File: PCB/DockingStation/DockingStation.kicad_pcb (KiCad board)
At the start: 4 copper layers, 147.2 x 63.2 mm, 256 parts, among them CN1 DSUB-15-HD_Socket_Horizontal_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, CN2 FDC_Connector, CN4 DSUB-25_Socket_Horizontal_P2.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, CN5 DSUB-9_Pins_Horizontal_P2.77x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, CN6 PS2 Connector, CN7 PS2 Connector, CN8 BarrelJack_Horizontal_PC110, J1 PCB Edge, J2 PCB Edge, J3 PCB Edge, J4 PCB Edge, Q1 3P4J, Q2 8C, U1 74VHCT244, U2 DNP (LT1237CS), U3 DS14C535MSA, U4 DNP

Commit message: Add files via upload
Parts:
- J1, J2, J3, J4: value PCB Edge -> 25-1MP_P0.5mm_Horizontal
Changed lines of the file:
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@@
 			)
 		)
-		(property "Value" "PCB Edge"
+		(property "Value" "25-1MP_P0.5mm_Horizontal"
 			(at 0 -3.25 0)
 			(layer "Dwgs.User")
@@
 			)
 		)
-		(property "Value" "PCB Edge"
+		(property "Value" "25-1MP_P0.5mm_Horizontal"
 			(at 0 -3.25 0)
 			(layer "Dwgs.User")
@@
 			)
 		)
-		(property "Value" "PCB Edge"
+		(property "Value" "25-1MP_P0.5mm_Horizontal"
 			(at 0 -3.25 0)
 			(layer "Dwgs.User")
@@
 			)
 		)
-		(property "Value" "PCB Edge"
+		(property "Value" "25-1MP_P0.5mm_Horizontal"
 			(at 0 -3.25 0)
 			(layer "Dwgs.User")

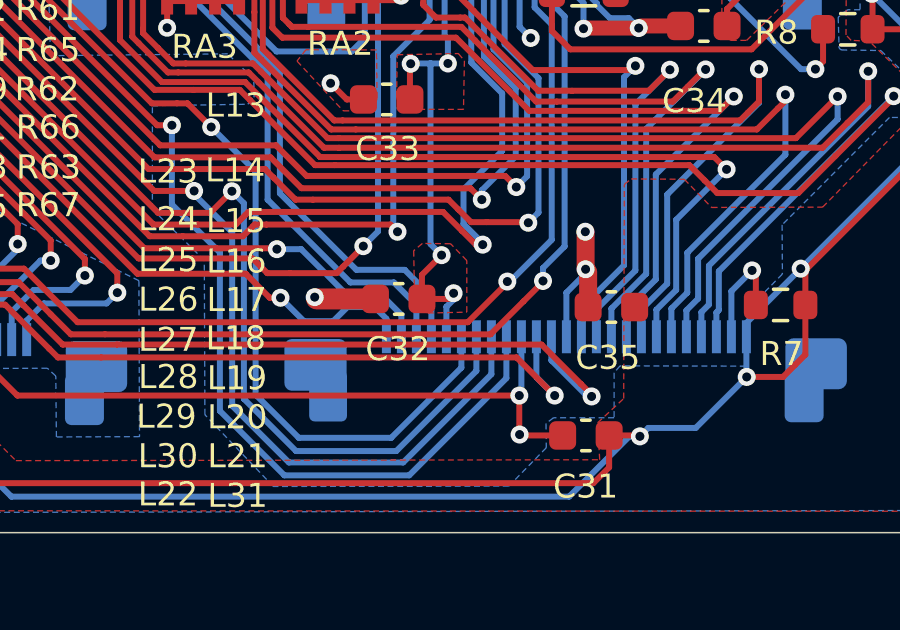
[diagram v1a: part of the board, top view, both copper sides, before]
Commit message: Add files via upload
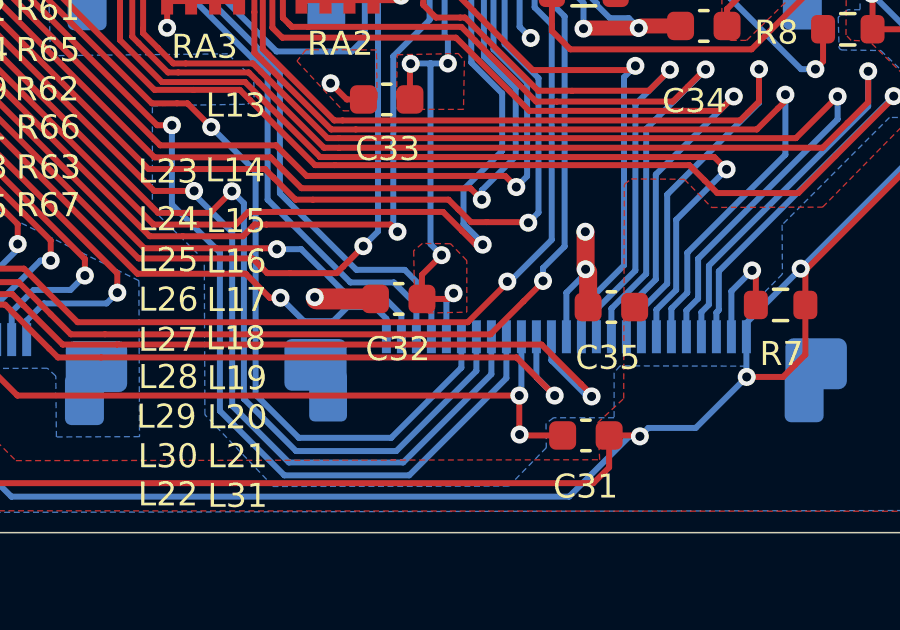
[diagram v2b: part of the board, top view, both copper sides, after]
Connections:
- net PNET1_Dock renamed PNET2
- net PNET2_Dock renamed PNET5
- C31 pad 2: (no net) -> PNET5_Q1_F2
- DA1 pad 3: (no net) -> VGA_RED
- DA2 pad 3: (no net) -> VGA_GREEN
- DA3 pad 3: (no net) -> VGA_BLUE
- J1 pad 11: (no net) -> VGA_BLUE
- J1 pad 13: (no net) -> R269_1_PC110
- J1 pad 14: (no net) -> M38_P16_R80_PC110
- J1 pad 15: (no net) -> M38_P67
- J1 pad 16: (no net) -> J13_60_PC110
- J1 pad 17: (no net) -> J13_59_PC110
- J1 pad 18: (no net) -> J13_58_PC110
- J1 pad 2: (no net) -> FDC_SLCTIN#
- J1 pad 24: (no net) -> J13_52_PC110
- J1 pad 3: (no net) -> FDC_AUTOFD#
- J1 pad 4: (no net) -> FDC_INIT#
- J1 pad 5: (no net) -> FDC_ACK#
- J1 pad 7: (no net) -> VGA_RED
- J1 pad 9: (no net) -> VGA_GREEN
- J2 pad 10: (no net) -> FDC_RDATA#
- J2 pad 11: (no net) -> J13_90_PC110
- J2 pad 14: (no net) -> KB_INT4
- J2 pad 15: (no net) -> KB_INT3
- J2 pad 17: (no net) -> FDC_DSR2#
- J2 pad 18: (no net) -> FDC_RTS2#
- J2 pad 19: (no net) -> FDC_CTS2#
- J2 pad 2: (no net) -> J13_99_PC110
- J2 pad 20: (no net) -> FDC_RI2#
- J2 pad 22: (no net) -> J13_79_PC110
- J2 pad 23: (no net) -> FDC_PE
- J2 pad 24: (no net) -> FDC_ERROR#
- J2 pad 25: (no net) -> FDC_PD6
- J2 pad 3: (no net) -> J13_98_PC110
- J2 pad 4: (no net) -> J13_97_PC110
- J2 pad 5: (no net) -> FDC_MEDIA2
- J2 pad 6: (no net) -> J13_95_PC110
- J2 pad 7: (no net) -> FDC_STEP#
- J2 pad 8: (no net) -> FDC_WGATE#
- J2 pad 9: (no net) -> J13_92_PC110
- J3 pad 10: (no net) -> FDC_WRTPRT#
- J3 pad 11: (no net) -> FDC_HDSEL#
- J3 pad 12: (no net) -> FDC_DSKCHG#
- J3 pad 14: (no net) -> KB_INT1
- J3 pad 15: (no net) -> KB_INT2
- J3 pad 16: (no net) -> PNET5_Q1_F2
- J3 pad 17: (no net) -> FDC_DCD2#
- J3 pad 18: (no net) -> U29_A2_FDC_IRRX_RXD2_InBuff
- J3 pad 19: (no net) -> U29_Y1_FDC_IRTX_TXD2_BufSW
- J3 pad 2: (no net) -> J13_2_PC110
- J3 pad 20: (no net) -> FDC_DTR2#
- J3 pad 22: (no net) -> FDC_BUSY
- J3 pad 23: (no net) -> FDC_SLCT
- J3 pad 24: (no net) -> FDC_PD7
- J3 pad 25: (no net) -> FDC_PD5
- J3 pad 3: (no net) -> FDC_MEDIA
- J3 pad 4: (no net) -> FDC_INDEX#
- J3 pad 5: (no net) -> FDC_DS0#
- J3 pad 6: (no net) -> FDC_MTR0#
- J3 pad 7: (no net) -> FDC_DIR#
- J3 pad 8: (no net) -> FDC_WDATA#
- J3 pad 9: (no net) -> FDC_TRK0
- J4 pad 1: (no net) -> FDC_PD4
- J4 pad 10: (no net) -> J13_35_PC110
- J4 pad 11: (no net) -> VGA_Hsync
- J4 pad 12: (no net) -> J13_37_PC110
- J4 pad 13: (no net) -> M38_P46_P34
- J4 pad 14: (no net) -> M38_P46_P34
- J4 pad 16: (no net) -> J13_41_PC110
- J4 pad 17: (no net) -> J13_42_PC110
- J4 pad 18: (no net) -> J13_43_PC110
- J4 pad 2: (no net) -> FDC_PD3
- J4 pad 24: (no net) -> J13_49_PC110
- J4 pad 3: (no net) -> FDC_PD2
- J4 pad 4: (no net) -> FDC_PD1
- J4 pad 5: (no net) -> FDC_PD0
- J4 pad 6: (no net) -> FDC_STROBE#
- J4 pad 7: (no net) -> J13_32_PC110
- J4 pad 8: (no net) -> VGA_Vsync
- J4 pad 9: (no net) -> J13_34_PC110
- L1 pad 1: (no net) -> VGA_GREEN
- L13 pad 1: (no net) -> FDC_MEDIA
- L14 pad 1: (no net) -> FDC_INDEX#
- L15 pad 1: (no net) -> FDC_DS0#
- L16 pad 1: (no net) -> FDC_MTR0#
- L17 pad 1: (no net) -> FDC_DIR#
- L18 pad 1: (no net) -> FDC_WDATA#
- L19 pad 1: (no net) -> FDC_TRK0
- L2 pad 1: (no net) -> VGA_BLUE
- L20 pad 1: (no net) -> FDC_WRTPRT#
- L21 pad 1: (no net) -> FDC_HDSEL#
- L22 pad 1: (no net) -> FDC_DSKCHG#
- L23 pad 1: (no net) -> J13_98_PC110
- L24 pad 1: (no net) -> J13_97_PC110
- L25 pad 1: (no net) -> FDC_MEDIA2
- L26 pad 1: (no net) -> J13_95_PC110
- L27 pad 1: (no net) -> FDC_STEP#
- L28 pad 1: (no net) -> FDC_WGATE#
- L29 pad 1: (no net) -> J13_92_PC110
- L3 pad 1: (no net) -> VGA_RED
- L31 pad 2: (no net) -> J13_90_PC110
- L38 pad 2: (no net) -> PNET5_Q1_F2
- L39 pad 2: (no net) -> KB_INT3
- L40 pad 2: (no net) -> KB_INT2
- L41 pad 2: (no net) -> KB_INT4
- L42 pad 2: (no net) -> KB_INT1
- Q2 pad 3: (no net) -> M38_P46_P34
- R12 pad 1: (no net) -> FDC_PD7
- R13 pad 1: (no net) -> FDC_PD5
- R14 pad 1: (no net) -> FDC_PD3
- R15 pad 1: (no net) -> FDC_PD1
- R16 pad 1: (no net) -> FDC_STROBE#
- R17 pad 1: (no net) -> FDC_INIT#
- R18 pad 1: (no net) -> FDC_SLCT
- R19 pad 1: (no net) -> FDC_ERROR#
- R20 pad 1: (no net) -> FDC_BUSY
- R21 pad 2: (no net) -> FDC_PD6
- R22 pad 1: (no net) -> FDC_PD4
- R23 pad 1: (no net) -> FDC_PD2
- R24 pad 1: (no net) -> FDC_PD0
- R25 pad 1: (no net) -> FDC_AUTOFD#
- R26 pad 1: (no net) -> FDC_SLCTIN#
- R27 pad 1: (no net) -> FDC_PE
- R28 pad 1: (no net) -> FDC_ACK#
- R3 pad 1: (no net) -> VGA_Hsync
- R33 pad 1: (no net) -> M38_P67
- R34 pad 2: (no net) -> M38_P67
- R38 pad 1: (no net) -> R269_1_PC110
- R4 pad 1: (no net) -> VGA_Vsync
- R41 pad 1: (no net) -> J13_79_PC110
- R43 pad 2: (no net) -> J13_79_PC110
- R44 pad 2: (no net) -> FDC_DTR2#
- R45 pad 2: (no net) -> U29_Y1_FDC_IRTX_TXD2_BufSW
- R46 pad 2: (no net) -> FDC_CTS2#
- R47 pad 2: (no net) -> U29_A2_FDC_IRRX_RXD2_InBuff
- R49 pad 2: (no net) -> FDC_DCD2#
- R50 pad 2: (no net) -> FDC_DSR2#
- R51 pad 1: (no net) -> FDC_RI2#
- R52 pad 1: (no net) -> FDC_DTR2#
- R54 pad 1: (no net) -> U29_Y1_FDC_IRTX_TXD2_BufSW
- R55 pad 1: (no net) -> FDC_DCD2#
- R56 pad 1: (no net) -> FDC_CTS2#
- R57 pad 1: (no net) -> FDC_DSR2#
- R58 pad 1: (no net) -> U29_A2_FDC_IRRX_RXD2_InBuff
- R59 pad 2: (no net) -> FDC_RI2#
- R7 pad 1: (no net) -> J13_2_PC110
- R8 pad 1: (no net) -> J13_99_PC110
- R9 pad 1: (no net) -> FDC_CTS2#
- RA2 pad 5: (no net) -> FDC_DSKCHG#
- RA2 pad 6: (no net) -> FDC_HDSEL#
- RA2 pad 8: (no net) -> FDC_WRTPRT#
- RA3 pad 6: (no net) -> FDC_MTR0#
- RA3 pad 7: (no net) -> FDC_DS0#
- RA3 pad 8: (no net) -> FDC_INDEX#
- RA4 pad 5: (no net) -> FDC_TRK0
- RA4 pad 6: (no net) -> FDC_WGATE#
- RA4 pad 7: (no net) -> FDC_WDATA#
- RA4 pad 8: (no net) -> FDC_STEP#
- RA5 pad 5: (no net) -> J13_92_PC110
- RA5 pad 6: (no net) -> FDC_DIR#
- RA5 pad 7: (no net) -> J13_95_PC110
- RA6 pad 5: (no net) -> FDC_MEDIA2
- RA6 pad 6: (no net) -> J13_97_PC110
- RA6 pad 7: (no net) -> J13_98_PC110
- RA6 pad 8: (no net) -> FDC_MEDIA
- RA7 pad 5: (no net) -> FDC_PD7
- RA7 pad 6: (no net) -> FDC_PD6
- RA7 pad 7: (no net) -> FDC_PD5
- RA7 pad 8: (no net) -> FDC_PD4
- RA8 pad 5: (no net) -> FDC_PD3
- RA8 pad 6: (no net) -> FDC_PD2
- RA8 pad 7: (no net) -> FDC_PD1
- RA8 pad 8: (no net) -> FDC_PD0
- ZD4 pad 1: (no net) -> M38_P67
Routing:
- net (no net): track 5439.2 -> 1658.9 mm, vias 126 -> 44
- net KB_INT4: track 0.00 -> 128.9 mm, vias 0 -> 3
- net KB_INT3: track 0.00 -> 126.4 mm, vias 0 -> 3
- net PNET5_Q1_F2: track 0.00 -> 125.7 mm, vias 0 -> 6
- net KB_INT1: track 0.00 -> 123.0 mm, vias 0 -> 3
- net KB_INT2: track 0.00 -> 122.6 mm, vias 0 -> 3
- net M38_P46_P34: track 0.00 -> 112.3 mm, vias 0 -> 1
- net VGA_RED: track 0.00 -> 99.2 mm, vias 0 -> 1
- net FDC_ERROR#: track 0.00 -> 98.9 mm, vias 0 -> 1
- net FDC_PD6: track 0.00 -> 94.9 mm, vias 0 -> 1
- net VGA_GREEN: track 0.00 -> 94.3 mm, vias 0 -> 1
- net VGA_BLUE: track 0.00 -> 89.2 mm, vias 0 -> 1
- net FDC_PD7: track 0.00 -> 86.1 mm, vias 0 -> 1
- net FDC_PD5: track 0.00 -> 78.9 mm, vias 0 -> 1
- net VGA_Hsync: track 0.00 -> 78.8 mm, vias 0 -> 1
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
